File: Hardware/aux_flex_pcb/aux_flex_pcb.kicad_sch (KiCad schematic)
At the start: 11 parts, among them IC1 ICM-42688-P, J1 503552-0622, U1 BMP581

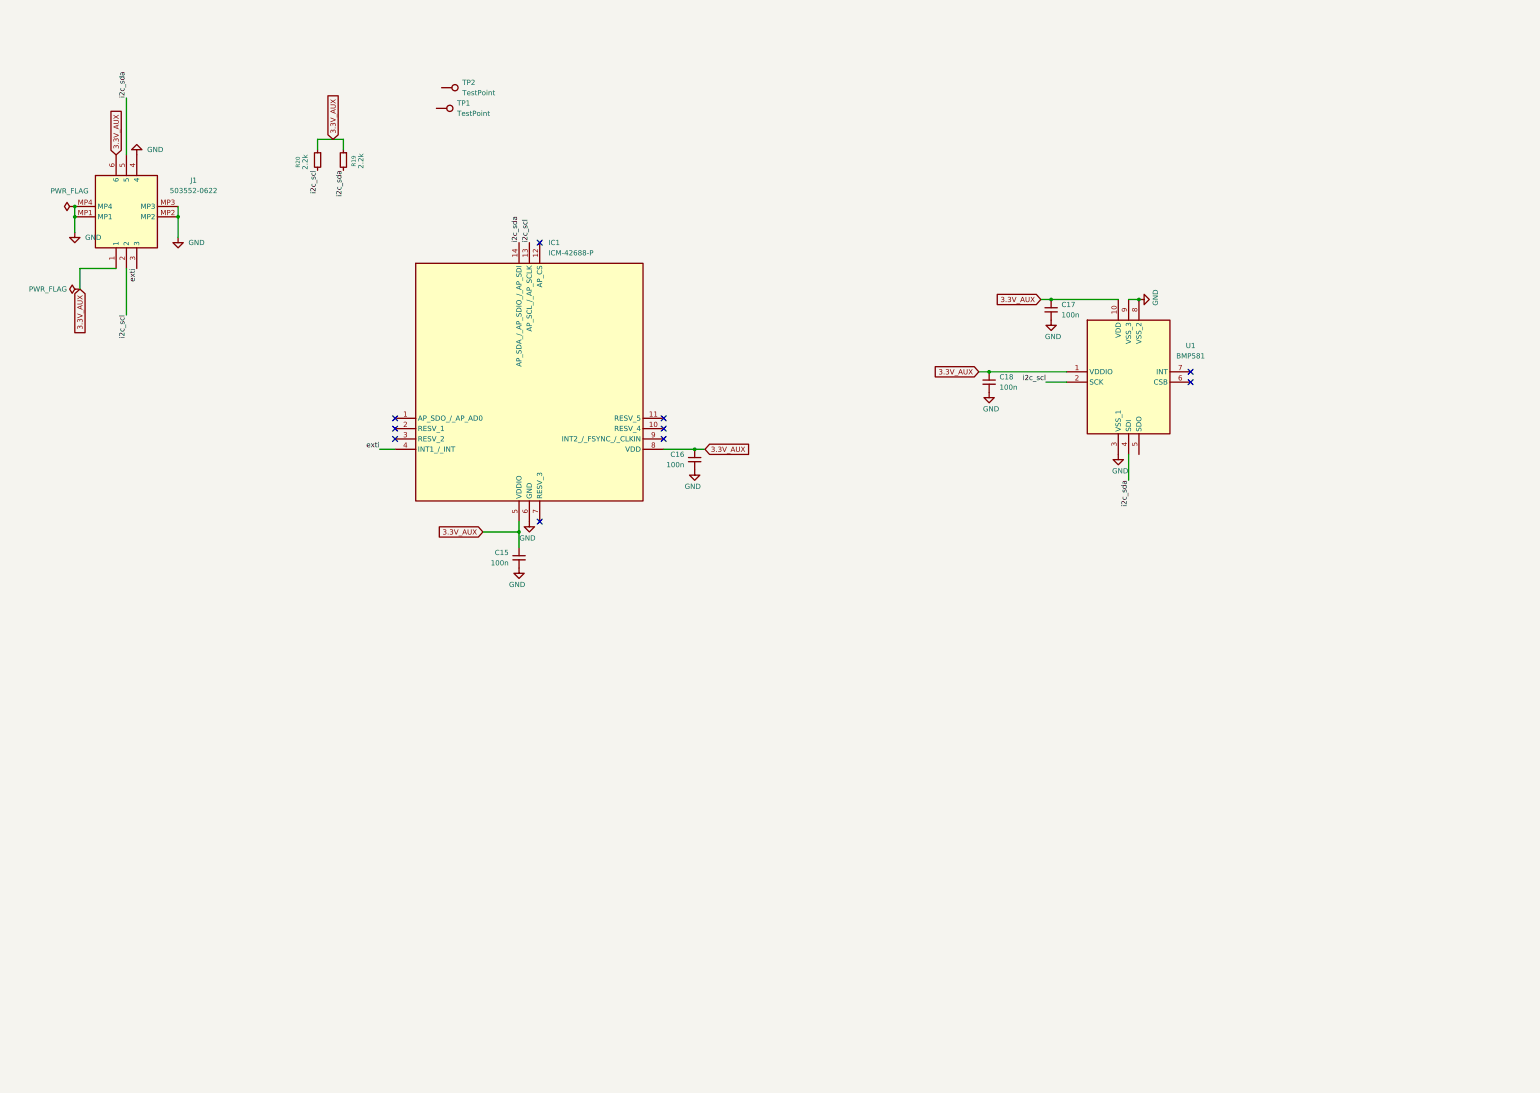
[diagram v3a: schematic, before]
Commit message: up
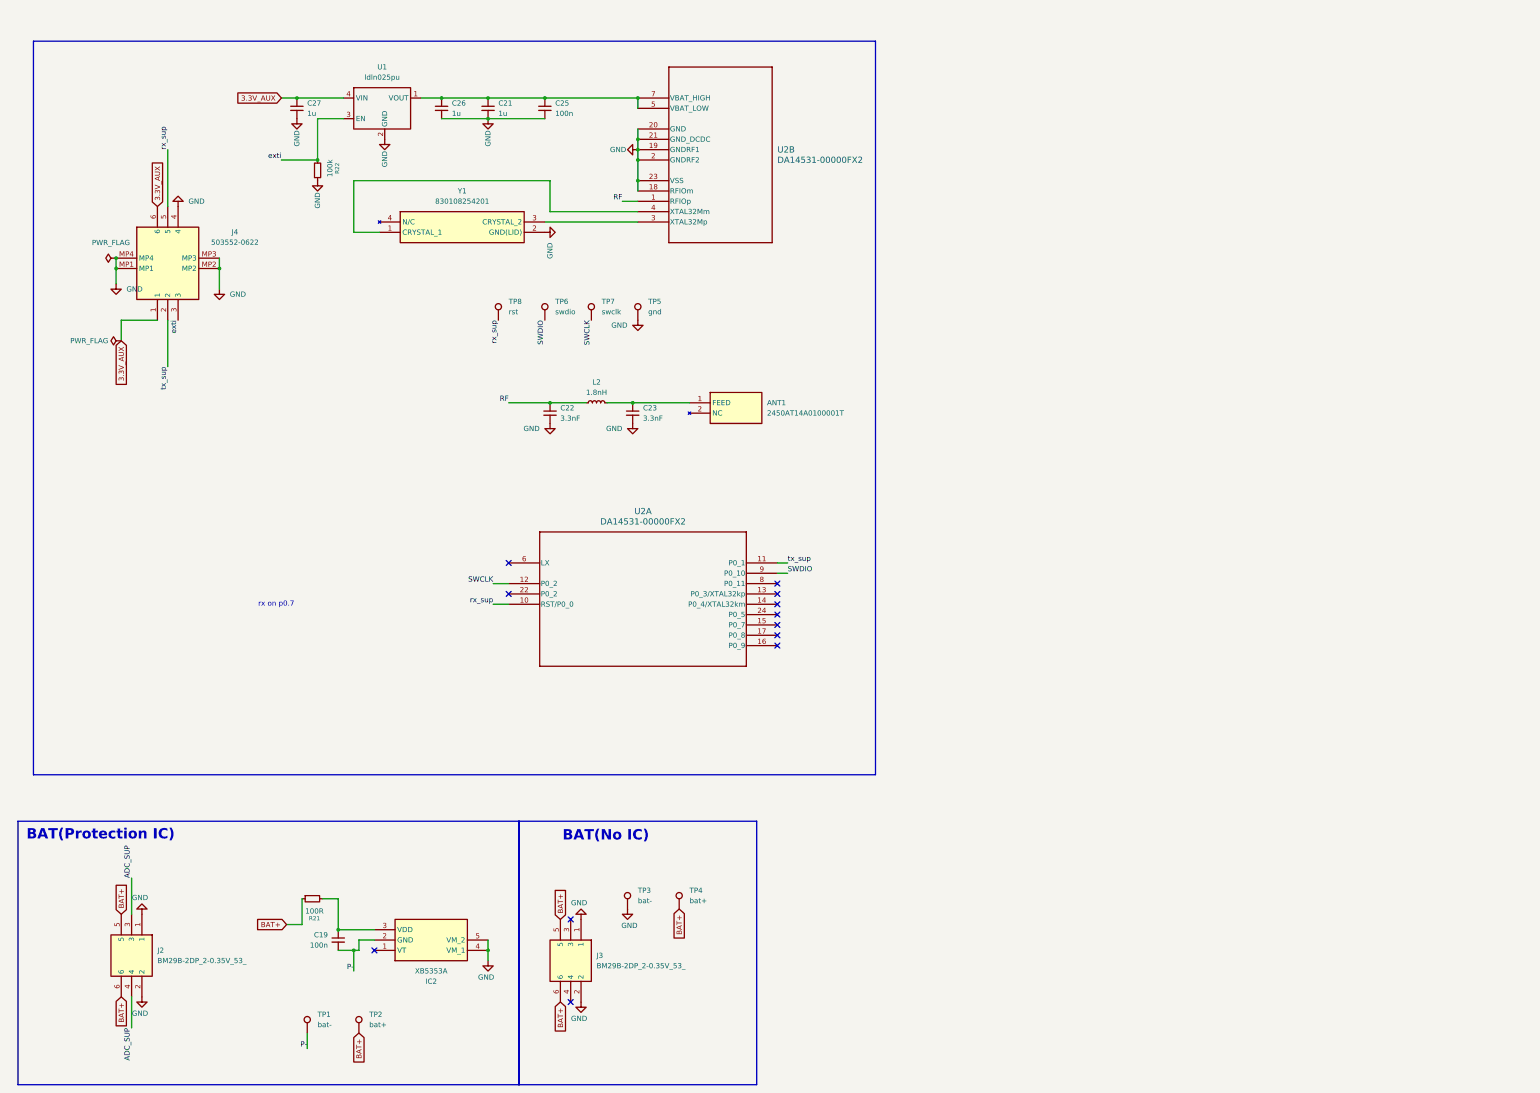
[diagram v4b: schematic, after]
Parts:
- removed C15, C16, C17, C18: 100n, Capacitor_SMD:C_0201_0603Metric_Pad0.64x0.40mm_HandSolder, symbol Device:C_Small
- removed IC1: ICM-42688-P, IIM42352, symbol samacsys:ICM-42688-P
- removed J1: 503552-0622, samacsys2:5035520622, symbol samacsys2:503552-0622
- removed R19, R20: 2.2k, Resistor_SMD:R_0201_0603Metric_Pad0.64x0.40mm_HandSolder, symbol Device:R_Small
- removed U1: BMP581, BMP581, symbol samacsys:BMP581
- added ANT1: 2450AT14A0100001T, samacsys2:2450AT14A0100001T, symbol samacsys2:2450AT14A0100001T
- added C19, C25: 100n, Capacitor_SMD:C_0201_0603Metric_Pad0.64x0.40mm_HandSolder, symbol Device:C_Small
- added C21, C26, C27: 1u, Capacitor_SMD:C_0201_0603Metric_Pad0.64x0.40mm_HandSolder, symbol Device:C_Small
- added C22, C23: 3.3nF, Capacitor_SMD:C_0201_0603Metric_Pad0.64x0.40mm_HandSolder, symbol Device:C_Small
- added IC2: XB5353A, samacsys2:SOT95P280X125-5N, symbol samacsys2:XB5353A
- added J2, J3: BM29B-2DP_2-0.35V_53_, samacsys2:BM29B2DP2035V53, symbol samacsys2:BM29B-2DP_2-0.35V_53_
- added J4: 503552-0622, samacsys2:5035520622, symbol samacsys2:503552-0622
- added L2: 1.8nH, Inductor_SMD:L_0201_0603Metric_Pad0.64x0.40mm_HandSolder, symbol Device:L_Small
- added R21: 100R, Resistor_SMD:R_0201_0603Metric_Pad0.64x0.40mm_HandSolder, symbol Device:R_Small
- added R22: 100k, Resistor_SMD:R_0201_0603Metric_Pad0.64x0.40mm_HandSolder, symbol Device:R_Small
- added TP3: bat-, symbol Connector:TestPoint
- added TP4: bat+, symbol Connector:TestPoint
- added TP5: gnd, samacsys2:1mm_circle, symbol Connector:TestPoint
- added TP6: swdio, samacsys2:1mm_circle, symbol Connector:TestPoint
- added TP7: swclk, samacsys2:1mm_circle, symbol Connector:TestPoint
- added TP8: rst, samacsys2:1mm_circle, symbol Connector:TestPoint
- added U1: ldln025pu, samacsys:ldln025pu, symbol samacsys:ldln025pu
- added U2: DA14531-00000FX2, samacsys2:FCGQFN24_2.2X3.0_REN, symbol samacsys2:DA14531-00000FX2
- added Y1: 830108254201, samacsys2:830108254201, symbol samacsys2:830108254201
- TP1: value TestPoint -> bat-; footprint samacsys2:1mm_circle -> (none)
- TP2: value TestPoint -> bat+; footprint samacsys2:1mm_circle -> (none)
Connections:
- net 3.3V_AUX: now also C27.1, J4.1, J4.6, U1.4 (VIN)
- net GND: now also C21.2, C22.2, C23.2, C25.2, C26.2, C27.2, IC2.4 (VM_1), IC2.5 (VM_2), J2.1, J2.2, J3.1, J3.2, J4.4, J4.MP1, J4.MP2, J4.MP3, J4.MP4, R22.1, TP3.1, TP5.1, U1.2 (GND), U2.18 (RFIOm), U2.19 (GNDRF1), U2.2 (GNDRF2), U2.20 (GND), U2.21 (GND_DCDC), U2.23 (VSS), Y1.2 (GND(LID))
- net exti: now also J4.3, R22.2, U1.3 (EN)
- net P-: now reaches TP1.1
- net P-: now also C19.2, IC2.2 (GND)
- net BAT+: now reaches TP2.1
- net BAT+: now also J2.5, J2.6, J3.5, J3.6, R21.1, TP4.1
- new net: C19.1, IC2.3 (VDD), R21.2
- new net: U2.3 (XTAL32Mp), Y1.3 (CRYSTAL_2)
- new net: U2.4 (XTAL32Mm), Y1.1 (CRYSTAL_1)
- new net: C21.1, C25.1, C26.1, U1.1 (VOUT), U2.5 (VBAT_LOW), U2.7 (VBAT_HIGH)
- new net: ANT1.1 (FEED), C23.1, L2.2
- new net ADC_SUP: J2.3, J2.4
- new net RF: C22.1, L2.1, U2.1 (RFIOp)
- new net SWCLK: TP7.1, U2.12 (P0_2)
- new net SWDIO: TP6.1, U2.9 (P0_10)
- new net rx_sup: J4.5, TP8.1, U2.10 (RST/P0_0)
- new net tx_sup: J4.2, U2.11 (P0_1)
- no-connect marks 10 -> 12
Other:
- note added: "BAT(No IC)"
- note added: "BAT(Protection IC)"
- note added: "rx on p0.7"
